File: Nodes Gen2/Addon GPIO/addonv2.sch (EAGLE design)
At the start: 55 parts

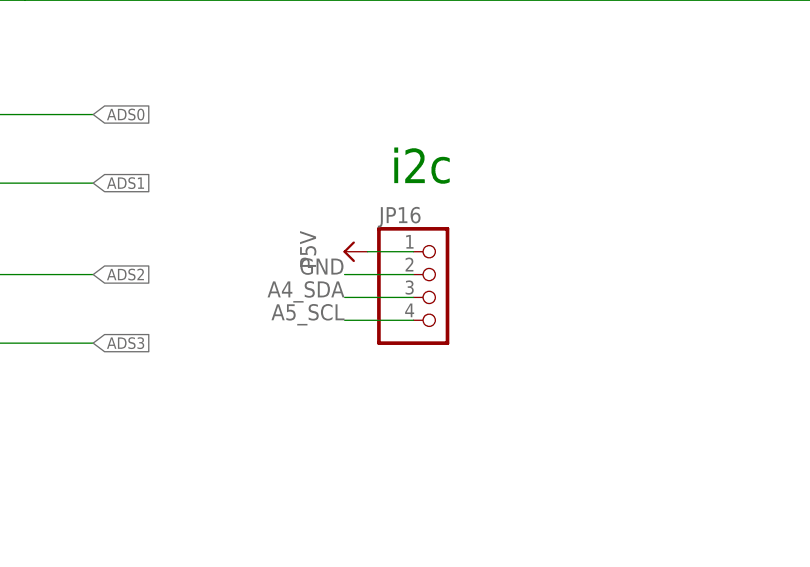
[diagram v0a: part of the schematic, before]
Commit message: so much...
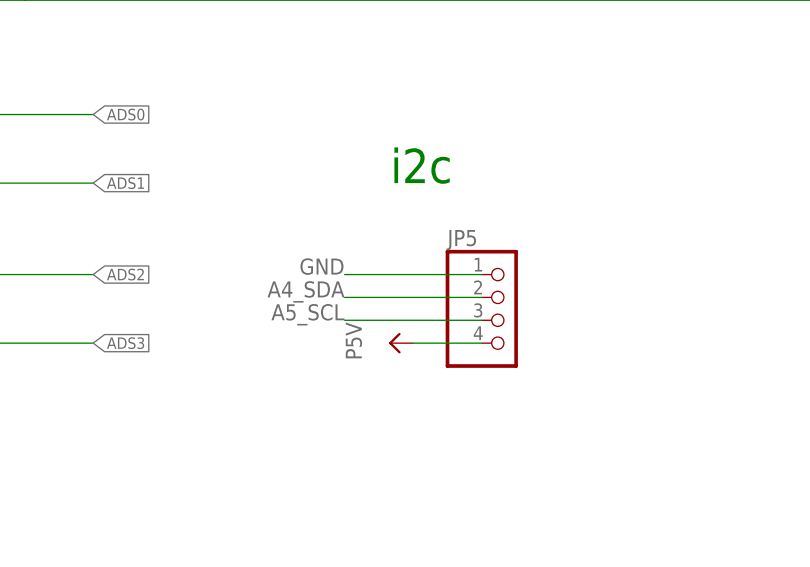
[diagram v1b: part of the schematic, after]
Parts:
- removed JP16: (no value), pinhead:PINHD-1X4/90
- added JP5: (no value), pinhead:PINHD-1X4/90
- R1, R17, R18, R19, R2, R20, R21, R22, R23, R24, R25, R26, R27, R28, R29, R3, R30, R31, R4, R5, R6, R7, R8: device rcl:R-EU_R0805 -> debauer_passiv:R-EU_R0603
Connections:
- net A4_SDA: now also JP5.2; no longer JP16.3
- net A5_SCL: now also JP5.3; no longer JP16.4
- net GND: now also JP5.1; no longer JP16.2
- net P5V: now also JP5.4; no longer JP16.1
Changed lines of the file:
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@@
 <part name="U$1" library="schlager_ics" deviceset="MCP23S17-E/SO" device=""/>
 <part name="LED2" library="led" deviceset="LED" device="CHIPLED_0805" value="green"/>
-<part name="R1" library="rcl" deviceset="R-EU_" device="R0805" value="120"/>
+<part name="R1" library="debauer_passiv" deviceset="R-EU_" device="R0603" value="120"/>
 <part name="LED4" library="led" deviceset="LED" device="CHIPLED_0805" value="green"/>
-<part name="R2" library="rcl" deviceset="R-EU_" device="R0805" value="120"/>
+<part name="R2" library="debauer_passiv" deviceset="R-EU_" device="R0603" value="120"/>
 <part name="LED6" library="led" deviceset="LED" device="CHIPLED_0805" value="green"/>
-<part name="R3" library="rcl" deviceset="R-EU_" device="R0805" value="120"/>
+<part name="R3" library="debauer_passiv" deviceset="R-EU_" device="R0603" value="120"/>
 <part name="LED8" library="led" deviceset="LED" device="CHIPLED_0805" value="green"/>
-<part name="R4" library="rcl" deviceset="R-EU_" device="R0805" value="120"/>
+<part name="R4" library="debauer_passiv" deviceset="R-EU_" device="R0603" value="120"/>
 <part name="LED10" library="led" deviceset="LED" device="CHIPLED_0805" value="green"/>
-<part name="R5" library="rcl" deviceset="R-EU_" device="R0805" value="120"/>
+<part name="R5" library="debauer_passiv" deviceset="R-EU_" device="R0603" value="120"/>
 <part name="LED12" library="led" deviceset="LED" device="CHIPLED_0805" value="green"/>
-<part name="R6" library="rcl" deviceset="R-EU_" device="R0805" value="120"/>
+<part name="R6" library="debauer_passiv" deviceset="R-EU_" device="R0603" value="120"/>
 <part name="LED14" library="led" deviceset="LED" device="CHIPLED_0805" value="green"/>
-<part name="R7" library="rcl" deviceset="R-EU_" device="R0805" value="120"/>
+<part name="R7" library="debauer_passiv" deviceset="R-EU_" device="R0603" value="120"/>
 <part name="LED16" library="led" deviceset="LED" device="CHIPLED_0805" value="green"/>
-<part name="R8" library="rcl" deviceset="R-EU_" device="R0805" value="120"/>
+<part name="R8" library="debauer_passiv" deviceset="R-EU_" device="R0603" value="120"/>
 <part name="GND11" library="supply1" deviceset="GND" device=""/>
 <part name="GND12" library="supply1" deviceset="GND" device=""/>
@@
 <part name="SUPPLY9" library="schlager_supply" deviceset="P5V" device=""/>
 <part name="SUPPLY16" library="schlager_supply" deviceset="P5V" device=""/>
-<part name="R19" library="rcl" deviceset="R-EU_" device="R0805" value="10k"/>
-<part name="R20" library="rcl" deviceset="R-EU_" device="R0805" value="10k"/>
-<part name="R21" library="rcl" deviceset="R-EU_" device="R0805" value="10k"/>
-<part name="R22" library="rcl" deviceset="R-EU_" device="R0805" value="10k"/>
+<part name="R19" library="debauer_passiv" deviceset="R-EU_" device="R0603" value="10k"/>
+<part name="R20" library="debauer_passiv" deviceset="R-EU_" device="R0603" value="10k"/>
+<part name="R21" library="debauer_passiv" deviceset="R-EU_" device="R0603" value="10k"/>
+<part name="R22" library="debauer_passiv" deviceset="R-EU_" device="R0603" value="10k"/>
 <part name="GND4" library="supply1" deviceset="GND" device=""/>
 <part name="JP9" library="pinhead" deviceset="PINHD-2X4" device="/90"/>
-<part name="R17" library="rcl" deviceset="R-EU_" device="R0805" value="10k"/>
-<part name="R18" library="rcl" deviceset="R-EU_" device="R0805" value="10k"/>
+<part name="R17" library="debauer_passiv" deviceset="R-EU_" device="R0603" value="10k"/>
+<part name="R18" library="debauer_passiv" deviceset="R-EU_" device="R0603" value="10k"/>
 <part name="SUPPLY10" library="schlager_supply" deviceset="P5V" device=""/>
 <part name="SUPPLY12" library="schlager_supply" deviceset="P5V" device=""/>
@@
 <part name="GND9" library="supply1" deviceset="GND" device=""/>
 <part name="SUPPLY22" library="schlager_supply" deviceset="P5V" device=""/>
-<part name="R23" library="rcl" deviceset="R-EU_" device="R0805" value="10k"/>
-<part name="R24" library="rcl" deviceset="R-EU_" device="R0805" value="10k"/>
+<part name="R23" library="debauer_passiv" deviceset="R-EU_" device="R0603" value="10k"/>
+<part name="R24" library="debauer_passiv" deviceset="R-EU_" device="R0603" value="10k"/>
 <part name="SUPPLY23" library="schlager_supply" deviceset="P5V" device=""/>
 <part name="SUPPLY24" library="schlager_supply" deviceset="P5V" device=""/>
 <part name="GND13" library="supply1" deviceset="GND" device=""/>
-<part name="JP16" library="pinhead" deviceset="PINHD-1X4" device="/90"/>
 <part name="SJ25" library="jumper" deviceset="SJ" device="N"/>
 <part name="SJ26" library="jumper" deviceset="SJ" device="N"/>
@@
 <part name="JP1" library="pinhead" deviceset="PINHD-2X3" device="/90"/>
 <part name="JP3" library="pinhead" deviceset="PINHD-2X3" device="/90"/>
-<part name="R25" library="rcl" deviceset="R-EU_" device="R0805" value="10k"/>
-<part name="R26" library="rcl" deviceset="R-EU_" device="R0805" value="10k"/>
-<part name="R27" library="rcl" deviceset="R-EU_" device="R0805" value="10k"/>
+<part name="R25" library="debauer_passiv" deviceset="R-EU_" device="R0603" value="10k"/>
+<part name="R26" library="debauer_passiv" deviceset="R-EU_" device="R0603" value="10k"/>
+<part name="R27" library="debauer_passiv" deviceset="R-EU_" device="R0603" value="10k"/>
 <part name="SUPPLY1" library="schlager_supply" deviceset="P5V" device=""/>
-<part name="R28" library="rcl" deviceset="R-EU_" device="R0805" value="10k"/>
-<part name="R29" library="rcl" deviceset="R-EU_" device="R0805" value="10k"/>
+<part name="R28" library="debauer_passiv" deviceset="R-EU_" device="R0603" value="10k"/>
+<part name="R29" library="debauer_passiv" deviceset="R-EU_" device="R0603" value="10k"/>
 <part name="SUPPLY5" library="schlager_supply" deviceset="P5V" device=""/>
 <part name="SUPPLY7" library="schlager_supply" deviceset="P5V" device=""/>
@@
 <part name="GND1" library="supply1" deviceset="GND" device=""/>
 <part name="SUPPLY8" library="schlager_supply" deviceset="P5V" device=""/>
-<part name="R30" library="rcl" deviceset="R-EU_" device="R0805" value="10k"/>
-<part name="R31" library="rcl" deviceset="R-EU_" device="R0805" value="10k"/>
+<part name="R30" library="debauer_passiv" deviceset="R-EU_" device="R0603" value="10k"/>
+<part name="R31" library="debauer_passiv" deviceset="R-EU_" device="R0603" value="10k"/>
 <part name="SUPPLY30" library="schlager_supply" deviceset="P5V" device=""/>
 <part name="SUPPLY31" library="schlager_supply" deviceset="P5V" device=""/>
 <part name="GND5" library="supply1" deviceset="GND" device=""/>
+<part name="JP5" library="pinhead" deviceset="PINHD-1X4" device="/90"/>
 </parts>
 <sheets>
@@
 <instance part="GND18" gate="1" x="96.52" y="12.7"/>
 <instance part="SUPPLY4" gate="G$1" x="294.64" y="198.12" rot="R90"/>
-<instance part="SUPPLY6" gate="G$1" x="139.7" y="68.58" rot="R90"/>
+<instance part="SUPPLY6" gate="G$1" x="144.78" y="58.42" rot="R90"/>
 <instance part="SUPPLY9" gate="G$1" x="104.14" y="20.32" rot="R270"/>
 <instance part="SUPPLY16" gate="G$1" x="55.88" y="73.66" rot="R90"/>
@@
 <instance part="SUPPLY24" gate="G$1" x="327.66" y="218.44" rot="MR0"/>
 <instance part="GND13" gate="1" x="322.58" y="205.74" rot="R90"/>
-<instance part="JP16" gate="A" x="149.86" y="63.5"/>
 <instance part="SJ25" gate="1" x="121.92" y="210.82" rot="R90"/>
 <instance part="SJ26" gate="1" x="124.46" y="210.82" rot="R90"/>
@@
 <instance part="SUPPLY31" gate="G$1" x="327.66" y="251.46" rot="MR0"/>
 <instance part="GND5" gate="1" x="322.58" y="238.76" rot="R90"/>
+<instance part="JP5" gate="A" x="157.48" y="60.96"/>
 </instances>
 <busses>
@@
 </segment>
 <segment>
-<wire x1="147.32" y1="66.04" x2="139.7" y2="66.04" width="0.1524" layer="91"/>
+<wire x1="154.94" y1="66.04" x2="139.7" y2="66.04" width="0.1524" layer="91"/>
 <label x="139.7" y="66.04" size="1.778" layer="95" rot="MR0"/>
-<pinref part="JP16" gate="A" pin="2"/>
+<pinref part="JP5" gate="A" pin="1"/>
 </segment>
 <segment>
@@
 <segment>
 <pinref part="SUPPLY6" gate="G$1" pin="P5V"/>
-<pinref part="JP16" gate="A" pin="1"/>
-<wire x1="147.32" y1="68.58" x2="142.24" y2="68.58" width="0.1524" layer="91"/>
+<wire x1="154.94" y1="58.42" x2="147.32" y2="58.42" width="0.1524" layer="91"/>
+<pinref part="JP5" gate="A" pin="4"/>
 </segment>
 <segment>
@@
 </segment>
 <segment>
-<wire x1="147.32" y1="63.5" x2="139.7" y2="63.5" width="0.1524" layer="91"/>
+<wire x1="154.94" y1="63.5" x2="139.7" y2="63.5" width="0.1524" layer="91"/>
 <label x="139.7" y="63.5" size="1.778" layer="95" rot="MR0"/>
-<pinref part="JP16" gate="A" pin="3"/>
+<pinref part="JP5" gate="A" pin="2"/>
 </segment>
 <segment>
@@
 </segment>
 <segment>
-<wire x1="147.32" y1="60.96" x2="139.7" y2="60.96" width="0.1524" layer="91"/>
+<wire x1="154.94" y1="60.96" x2="139.7" y2="60.96" width="0.1524" layer="91"/>
 <label x="139.7" y="60.96" size="1.778" layer="95" rot="MR0"/>
-<pinref part="JP16" gate="A" pin="4"/>
-</segment>
-<segment>
+<pinref part="JP5" gate="A" pin="3"/>
+</segment>
+<segment>
